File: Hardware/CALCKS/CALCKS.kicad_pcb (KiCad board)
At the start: 2 copper layers, 68 parts, among them J1 Conn_02x03_Counter_Clockwise, J2 USB_B_Micro, J3 Conn_01x01_Male, J4 Conn_01x01_Male, SW1 SW_Push_Dual, SW10 SW_Push_Dual, SW11 SW_Push_Dual, SW12 SW_Push_Dual, SW13 SW_Push_Dual, SW14 SW_Push_Dual, SW15 SW_Push_Dual, SW16 SW_Push_Dual, SW17 SW_Push_Dual, SW18 SW_Push_Dual, SW19 SW_Push_Dual, SW2 SW_Push_Dual, SW20 SW_Push_Dual, SW21 SW_Push_Dual, SW22 SW_Push_Dual, SW23 SW_Push_Dual, SW24 SW_Push_Dual, SW25 SW_Push_Dual, SW26 SW_Push_Dual, SW27 SW_Push_Dual, SW28 SW_Push_Dual, SW29 SW_Push_Dual, SW3 SW_Push_Dual, SW30 SW_Push_Dual, SW31 SW_Push_Dual, SW32 SW_Push_Dual, SW33 SW_Push_Dual, SW34 SW_Push_Dual, SW35 SW_Push_Dual, SW36 SW_Push_Dual, SW37 SW_Push_Dual, SW38 SW_Push_Dual, SW39 SW_Push_Dual, SW4 SW_Push_Dual, SW40 SW_Push_Dual, SW5 SW_Push_Dual, SW6 SW_Push_Dual, SW7 SW_Push_Dual, SW8 SW_Push_Dual, SW9 SW_Push_Dual, U1 ATmega1284-AU, U2 MCP73831-2-OT, U3 AT24CS64-SSHM, U4 74HC164, Y1 16MHz

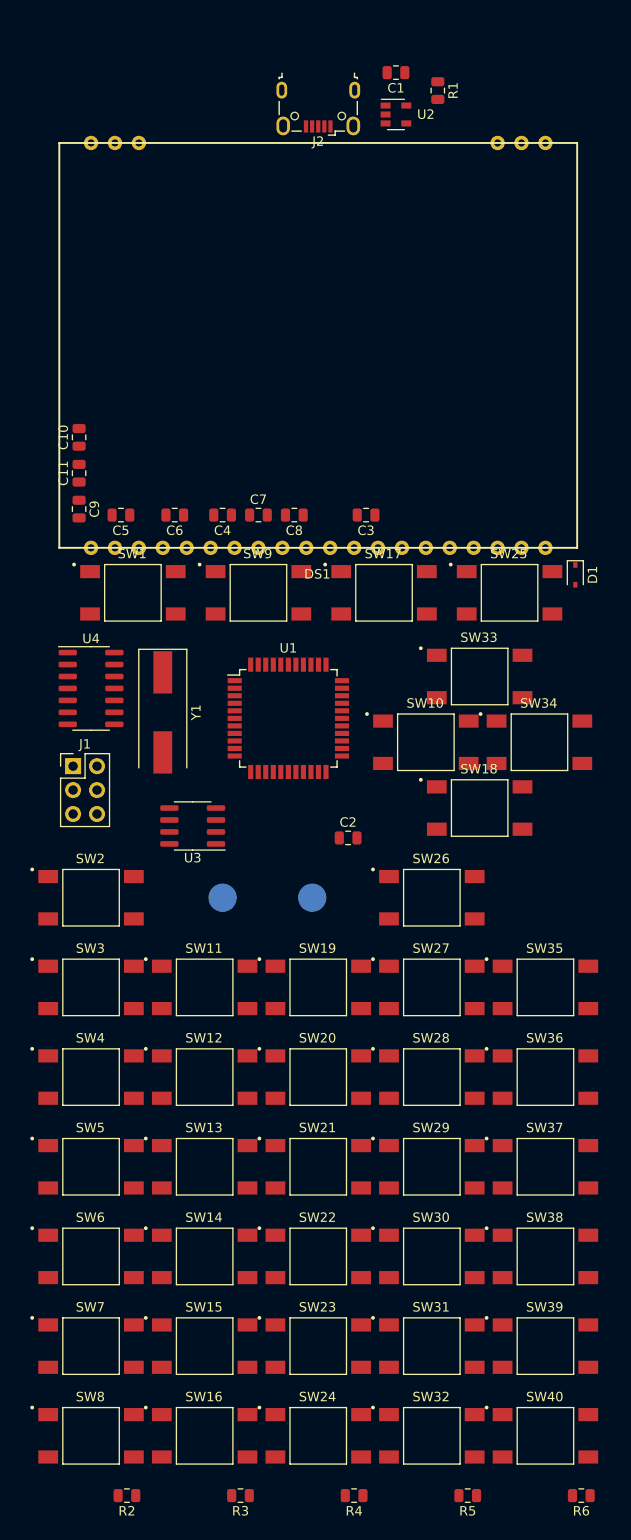
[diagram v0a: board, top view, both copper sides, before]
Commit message: Re-add version 2 of Hardware
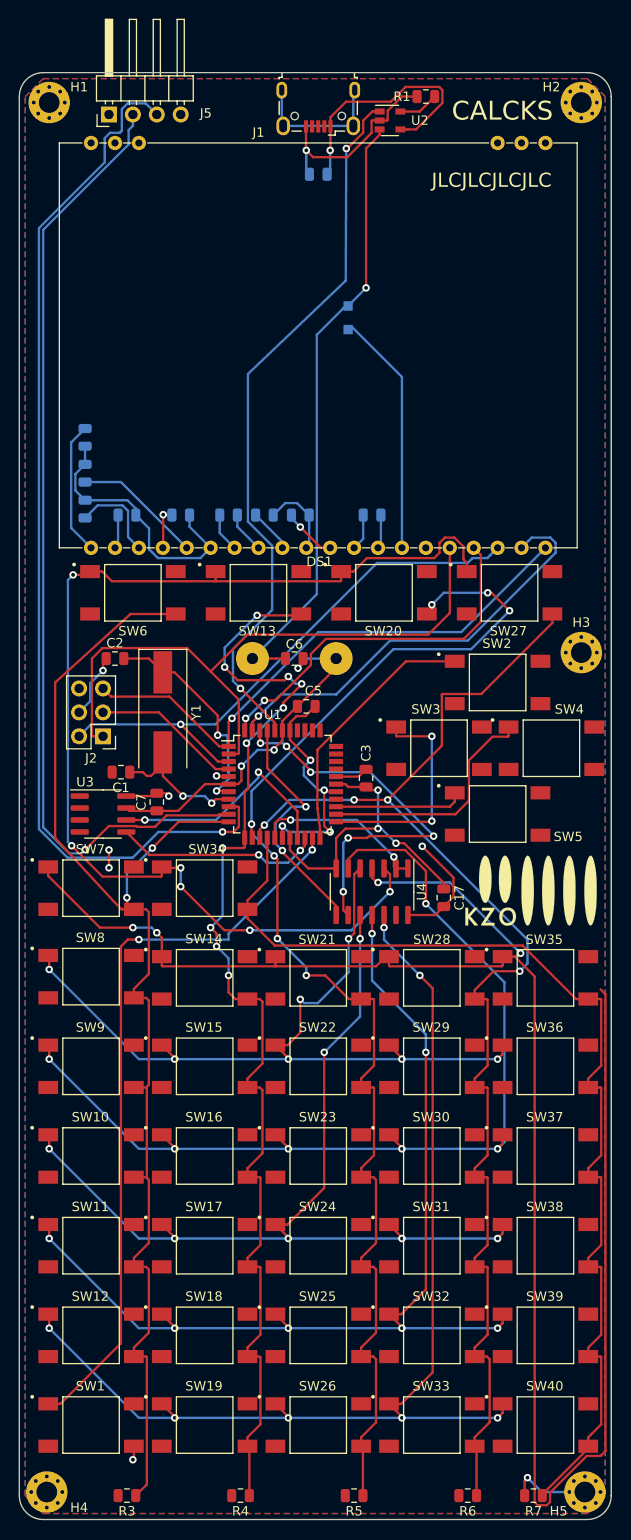
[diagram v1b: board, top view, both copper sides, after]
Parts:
- removed R2: 220, Resistor_SMD:R_0805_2012Metric
- added C17: 0.1uF, Capacitor_SMD:C_0805_2012Metric, F.Cu at (111.8, 113.7)
- added C2: 30pF, Capacitor_SMD:C_0805_2012Metric, F.Cu at (76.8, 88.3)
- added C3: 0.1uF, Capacitor_SMD:C_0805_2012Metric, F.Cu at (103.5, 101.0)
- added C4: 4.7uF, Capacitor_SMD:C_0805_2012Metric, B.Cu at (98.4, 36.8)
- added C5: 0.1uF, Capacitor_SMD:C_0805_2012Metric, F.Cu at (97.2, 93.3)
- added C7: 0.1uF, Capacitor_SMD:C_0805_2012Metric, F.Cu at (81.3, 103.5)
- added G***: LOGO, CALCKS:kzo_logo, F.Cu at (121.0, 112.9)
- added H1: MountingHole_Pad, MountingHole:MountingHole_2.2mm_M2_Pad_Via, F.Cu at (69.8, 29.2)
- added H2: MountingHole_Pad, MountingHole:MountingHole_2.2mm_M2_Pad_Via, F.Cu at (126.4, 29.2)
- added H3: MountingHole_Pad, MountingHole:MountingHole_2.2mm_M2_Pad_Via, F.Cu at (126.4, 87.6)
- added H4: MountingHole_Pad, MountingHole:MountingHole_2.2mm_M2_Pad_Via, F.Cu at (69.6, 176.8)
- added H5: MountingHole_Pad, MountingHole:MountingHole_2.2mm_M2_Pad_Via, F.Cu at (126.7, 176.8)
- added J5: Conn_01x04_Male, Connector_PinHeader_2.54mm:PinHeader_1x04_P2.54mm_Horizontal, F.Cu at (76.2, 30.5)
- added R3: 220, Resistor_SMD:R_0805_2012Metric, F.Cu at (78.1, 177.2)
- C1: value 4.7uF -> 30pF
- C10: renamed from C5; moved to B.Cu
- C11: renamed from C6; moved to B.Cu
- C12: renamed from C7; moved to B.Cu
- C13: renamed from C8; moved to B.Cu
- C14: renamed from C9; moved to B.Cu
- C15: renamed from C10; moved to B.Cu
- C16: renamed from C11; moved to B.Cu
- C8: renamed from C3; moved to B.Cu
- C9: renamed from C4; moved to B.Cu
- D1: footprint Diode_SMD:D_SOD-323 -> Diode_SMD:D_SOD-323_HandSoldering; moved to B.Cu
- J3, J4: footprint TestPoint:TestPoint_Pad_D3.0mm -> Connector_Wire:SolderWirePad_1x01_Drill1.2mm
- Y1: value 16MHz -> 8MHz
- moved SW2 85.8 mm to (117.5, 90.8)
- moved C1 79.8 mm to (77.5, 100.3)
- moved SW3 74.1 mm to (111.3, 97.8)
- moved SW4 74.1 mm to (123.2, 97.8)
- moved SW5 66.2 mm to (117.5, 104.8)
- moved SW34 38.8 mm to (86.4, 112.6)
- moved U4 36.8 mm to (104.1, 113.0), turned to 270 degrees
- moved D1 36.4 mm to (101.6, 52.1), turned to 90 degrees
- moved SW14 34.3 mm to (86.4, 122.2)
- moved SW35 32.8 mm to (122.6, 122.2)
- moved J3 28.1 mm to (100.3, 88.3)
- moved J4 26.2 mm to (91.4, 88.3)
- moved SW21 24.9 mm to (98.4, 122.2)
- moved C6 19.9 mm to (95.9, 88.3), turned to 180 degrees
- moved U3 9.61 mm to (75.6, 104.8), turned to 0 degrees
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- renumbered C2 to C6, J2 to J1, J1 to J2, R3 to R4, R4 to R5, R5 to R6, R6 to R7, SW8 to SW1, SW5 to SW10, SW6 to SW11, SW7 to SW12, SW9 to SW13, SW10 to SW14, SW11 to SW15, SW12 to SW16, SW13 to SW17, SW14 to SW18, SW15 to SW19, SW16 to SW2, SW17 to SW20, SW18 to SW21, SW19 to SW22, SW20 to SW23, SW21 to SW24, SW22 to SW25, SW23 to SW26, SW25 to SW27, SW26 to SW28, SW27 to SW29, SW24 to SW3, SW28 to SW30, SW29 to SW31, SW30 to SW32, SW31 to SW33, SW33 to SW35, SW35 to SW36, SW36 to SW37, SW37 to SW38, SW38 to SW39, SW32 to SW4, SW39 to SW40, SW40 to SW5, SW1 to SW6, SW2 to SW7, SW3 to SW8, SW4 to SW9
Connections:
- C1 pad 2: GND -> -BATT
- C10 pad 1: GND -> -BATT
- C11 pad 1: GND -> -BATT
- C14 pad 1: GND -> -BATT
- C15 pad 1: GND -> -BATT
- C16 pad 1: GND -> -BATT
- C6 pad 1: GND -> -BATT
- C6 pad 2: Net-(C2-Pad2) (its old number) -> +BATT
- C8 pad 1: GND -> -BATT
- D1 pad 2: Net-(C2-Pad2) (its old number) -> +BATT
- DS1 pad 26: GND -> -BATT
- DS1 pad 33: GND -> -BATT
- J1 pad 1: Net-(C1-Pad1) -> Net-(C4-Pad1)
- J1 pad 5: GND -> Net-(C4-Pad2)
- J2 pad 4: GND -> -BATT
- J3 pad 1: GND -> -BATT
- J4 pad 1: Net-(C2-Pad2) (its old number) -> +BATT
- R1 pad 1: GND -> Net-(C4-Pad2)
- R4 pad 2: GND -> -BATT
- R5 pad 2: GND -> -BATT
- R6 pad 2: GND -> -BATT
- R7 pad 2: GND -> -BATT
- SW1 pad 1: Net-(SW16-Pad1) (its old number) -> Net-(SW1-Pad1)
- SW1 pad 2: BTN_ROW1 -> Net-(SW1-Pad2)
- SW1 pad 4: Net-(SW8-Pad4) -> -BATT
- SW10 pad 2: BTN_ROW1 -> Net-(SW10-Pad2)
- SW10 pad 4: Net-(SW5-Pad4) -> BTN_ROW1
- SW11 pad 2: BTN_ROW1 -> Net-(SW11-Pad2)
- SW11 pad 4: Net-(SW6-Pad4) -> BTN_ROW1
- SW12 pad 2: BTN_ROW1 -> Net-(SW12-Pad2)
- SW12 pad 4: Net-(SW7-Pad4) -> BTN_ROW1
- SW13 pad 2: BTN_ROW2 -> Net-(SW13-Pad2)
- SW13 pad 4: Net-(SW9-Pad4) -> BTN_ROW2
- SW14 pad 2: BTN_ROW2 -> Net-(SW14-Pad2)
- SW14 pad 4: Net-(SW10-Pad4) -> BTN_ROW2
- SW15 pad 2: BTN_ROW2 -> Net-(SW15-Pad2)
- SW15 pad 4: Net-(SW11-Pad4) -> BTN_ROW2
- SW16 pad 2: BTN_ROW2 -> Net-(SW16-Pad2)
- SW16 pad 4: Net-(SW12-Pad4) -> BTN_ROW2
- SW17 pad 2: BTN_ROW2 -> Net-(SW17-Pad2)
- SW17 pad 4: Net-(SW13-Pad4) -> BTN_ROW2
- SW18 pad 2: BTN_ROW2 -> Net-(SW18-Pad2)
- SW18 pad 4: Net-(SW14-Pad4) -> BTN_ROW2
- SW19 pad 2: BTN_ROW2 -> Net-(SW19-Pad2)
- SW19 pad 4: Net-(SW15-Pad4) -> BTN_ROW2
- SW2 pad 1: Net-(SW16-Pad1) (its old number) -> Net-(SW2-Pad1)
- SW2 pad 2: BTN_ROW2 -> Net-(SW2-Pad2)
- SW2 pad 4: Net-(SW16-Pad4) -> -BATT
- SW20 pad 2: BTN_ROW3 -> Net-(SW20-Pad2)
- SW20 pad 4: Net-(SW17-Pad4) -> BTN_ROW3
- SW21 pad 2: BTN_ROW3 -> Net-(SW21-Pad2)
- SW21 pad 4: Net-(SW18-Pad4) -> BTN_ROW3
- SW22 pad 2: BTN_ROW3 -> Net-(SW22-Pad2)
- SW22 pad 4: Net-(SW19-Pad4) -> BTN_ROW3
- SW23 pad 2: BTN_ROW3 -> Net-(SW23-Pad2)
- SW23 pad 4: Net-(SW20-Pad4) -> BTN_ROW3
- SW24 pad 2: BTN_ROW3 -> Net-(SW24-Pad2)
- SW24 pad 4: Net-(SW21-Pad4) -> BTN_ROW3
- SW25 pad 2: BTN_ROW3 -> Net-(SW25-Pad2)
- SW25 pad 4: Net-(SW22-Pad4) -> BTN_ROW3
- SW26 pad 2: BTN_ROW3 -> Net-(SW26-Pad2)
- SW26 pad 4: Net-(SW23-Pad4) -> BTN_ROW3
- SW27 pad 2: BTN_ROW4 -> Net-(SW27-Pad2)
- SW27 pad 4: Net-(SW25-Pad4) -> BTN_ROW4
- SW28 pad 2: BTN_ROW4 -> Net-(SW28-Pad2)
- SW28 pad 4: Net-(SW26-Pad4) -> BTN_ROW4
- SW29 pad 2: BTN_ROW4 -> Net-(SW29-Pad2)
- SW29 pad 4: Net-(SW27-Pad4) -> BTN_ROW4
- SW3 pad 1: Net-(SW16-Pad1) (its old number) -> Net-(SW3-Pad1)
- SW3 pad 2: BTN_ROW3 -> Net-(SW3-Pad2)
- SW3 pad 4: Net-(SW24-Pad4) -> -BATT
- SW30 pad 2: BTN_ROW4 -> Net-(SW30-Pad2)
- SW30 pad 4: Net-(SW28-Pad4) -> BTN_ROW4
- SW31 pad 2: BTN_ROW4 -> Net-(SW31-Pad2)
- SW31 pad 4: Net-(SW29-Pad4) -> BTN_ROW4
- SW32 pad 2: BTN_ROW4 -> Net-(SW32-Pad2)
- SW32 pad 4: Net-(SW30-Pad4) -> BTN_ROW4
- SW33 pad 2: BTN_ROW4 -> Net-(SW33-Pad2)
- SW33 pad 4: Net-(SW31-Pad4) -> BTN_ROW4
- SW34 pad 2: BTN_ROW5 -> Net-(SW34-Pad2)
- SW34 pad 4: Net-(SW34-Pad4) -> BTN_ROW5
- SW35 pad 2: BTN_ROW5 -> Net-(SW35-Pad2)
- SW35 pad 4: Net-(SW33-Pad4) -> BTN_ROW5
- SW36 pad 2: BTN_ROW5 -> Net-(SW36-Pad2)
- SW36 pad 4: Net-(SW35-Pad4) -> BTN_ROW5
- SW37 pad 2: BTN_ROW5 -> Net-(SW37-Pad2)
- SW37 pad 4: Net-(SW36-Pad4) -> BTN_ROW5
- SW38 pad 2: BTN_ROW5 -> Net-(SW38-Pad2)
- SW38 pad 4: Net-(SW37-Pad4) -> BTN_ROW5
- SW39 pad 2: BTN_ROW5 -> Net-(SW39-Pad2)
- SW39 pad 4: Net-(SW38-Pad4) -> BTN_ROW5
- SW4 pad 1: Net-(SW16-Pad1) (its old number) -> Net-(SW4-Pad1)
- SW4 pad 2: BTN_ROW4 -> Net-(SW4-Pad2)
- SW4 pad 4: Net-(SW32-Pad4) -> -BATT
- SW40 pad 2: BTN_ROW5 -> Net-(SW40-Pad2)
- SW40 pad 4: Net-(SW39-Pad4) -> BTN_ROW5
- SW5 pad 1: Net-(SW16-Pad1) (its old number) -> Net-(SW5-Pad1)
- SW5 pad 2: BTN_ROW5 -> Net-(SW5-Pad2)
- SW5 pad 4: Net-(SW40-Pad4) -> -BATT
- SW6 pad 2: BTN_ROW1 -> Net-(SW6-Pad2)
- SW6 pad 4: Net-(SW1-Pad4) -> BTN_ROW1
- SW7 pad 2: BTN_ROW1 -> Net-(SW7-Pad2)
- SW7 pad 4: Net-(SW2-Pad4) -> BTN_ROW1
- SW8 pad 2: BTN_ROW1 -> Net-(SW8-Pad2)
- SW8 pad 4: Net-(SW3-Pad4) -> BTN_ROW1
- SW9 pad 2: BTN_ROW1 -> Net-(SW9-Pad2)
- SW9 pad 4: Net-(SW4-Pad4) -> BTN_ROW1
- U1 pad 10: BTN_ROW2 -> TXD0
- U1 pad 11: BTN_ROW3 -> BTN_ROW1
- U1 pad 12: BTN_ROW4 -> BTN_ROW2
- U1 pad 13: BTN_ROW5 -> BTN_ROW3
- U1 pad 14: CLK -> BTN_ROW4
- U1 pad 15: CLR -> BTN_ROW5
- U1 pad 18: GND -> -BATT
- U1 pad 21: Net-(U1-Pad21) -> Net-(SW1-Pad1)
- U1 pad 22: Net-(U1-Pad22) -> Net-(SW2-Pad1)
- U1 pad 23: Net-(U1-Pad23) -> Net-(SW3-Pad1)
- U1 pad 24: Net-(U1-Pad24) -> Net-(SW4-Pad1)
- U1 pad 25: Net-(U1-Pad25) -> Net-(SW5-Pad1)
- U1 pad 28: GND -> -BATT
- U1 pad 29: VCC -> Net-(C3-Pad2)
- U1 pad 39: GND -> -BATT
- U1 pad 41: Net-(U1-Pad41) -> CLK
- U1 pad 42: Net-(U1-Pad42) -> CLR
- U1 pad 6: GND -> -BATT
- U1 pad 8: Net-(U1-Pad8) -> Net-(C1-Pad1)
- U1 pad 9: BTN_ROW1 -> RXD0
- U2 pad 2: GND -> Net-(C4-Pad2)
- U2 pad 3: Net-(C2-Pad2) (its old number) -> +BATT
- U2 pad 4: Net-(C1-Pad1) -> Net-(C4-Pad1)
- U3 pad 1: GND -> -BATT
- U3 pad 2: GND -> -BATT
- U3 pad 3: GND -> -BATT
- U3 pad 4: GND -> -BATT
- U3 pad 7: GND -> -BATT
- U4 pad 13: Net-(SW16-Pad1) (its old number) -> Net-(U4-Pad13)
- U4 pad 7: GND -> -BATT
- Y1 pad 2: Net-(U1-Pad8) -> Net-(C1-Pad1)
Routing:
- net Net-(SW14-Pad1): track 0.00 -> 199.1 mm, vias 0 -> 4
- net BTN_ROW3: track 0.00 -> 139.3 mm, vias 0 -> 7
- net BTN_ROW4: track 0.00 -> 138.9 mm, vias 0 -> 4
- net BTN_ROW1: track 0.00 -> 134.2 mm, vias 0 -> 2
- net BTN_ROW2: track 0.00 -> 125.1 mm, vias 0 -> 10
- net -BATT: track 0.00 -> 123.4 mm, vias 0 -> 9
- net Net-(SW13-Pad1): track 0.00 -> 123.0 mm, vias 0 -> 6
- net Net-(SW12-Pad1): track 0.00 -> 117.7 mm, vias 0 -> 7
- net BTN_ROW5: track 0.00 -> 113.3 mm
- net RXD0: track 0.00 -> 112.2 mm, vias 0 -> 1
- net Net-(SW11-Pad1): track 0.00 -> 108.1 mm, vias 0 -> 7
- net Net-(SW16-Pad1): track 0.00 -> 104.8 mm, vias 0 -> 6
- net TXD0: track 0.00 -> 102.3 mm, vias 0 -> 1
- net Net-(SW10-Pad1): track 0.00 -> 98.3 mm, vias 0 -> 7
- net Net-(SW15-Pad1): track 0.00 -> 85.9 mm, vias 0 -> 7
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- added copper zone on F.Cu, net -BATT
- added copper zone on B.Cu, net VCC
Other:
- board outline added: 62.9 x 153.7 mm
- board text added: "CALCKS"
- board text added: "JLCJLCJLCJLC"
